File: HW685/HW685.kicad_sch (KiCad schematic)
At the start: 15 parts, among them J1 Screw_Terminal_01x03, J2 Screw_Terminal_01x02, U1 ICL7660, U2 LM358

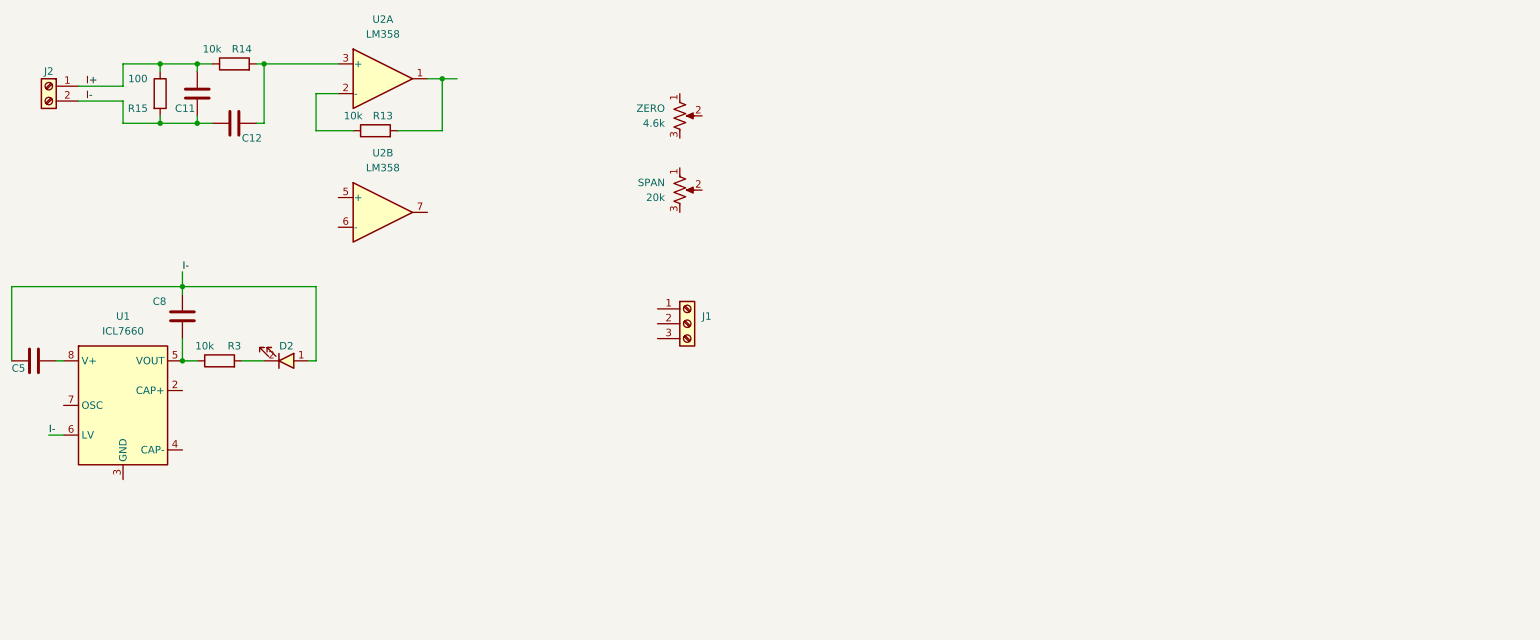
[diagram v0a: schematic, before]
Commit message: Complete HW685 Schematic
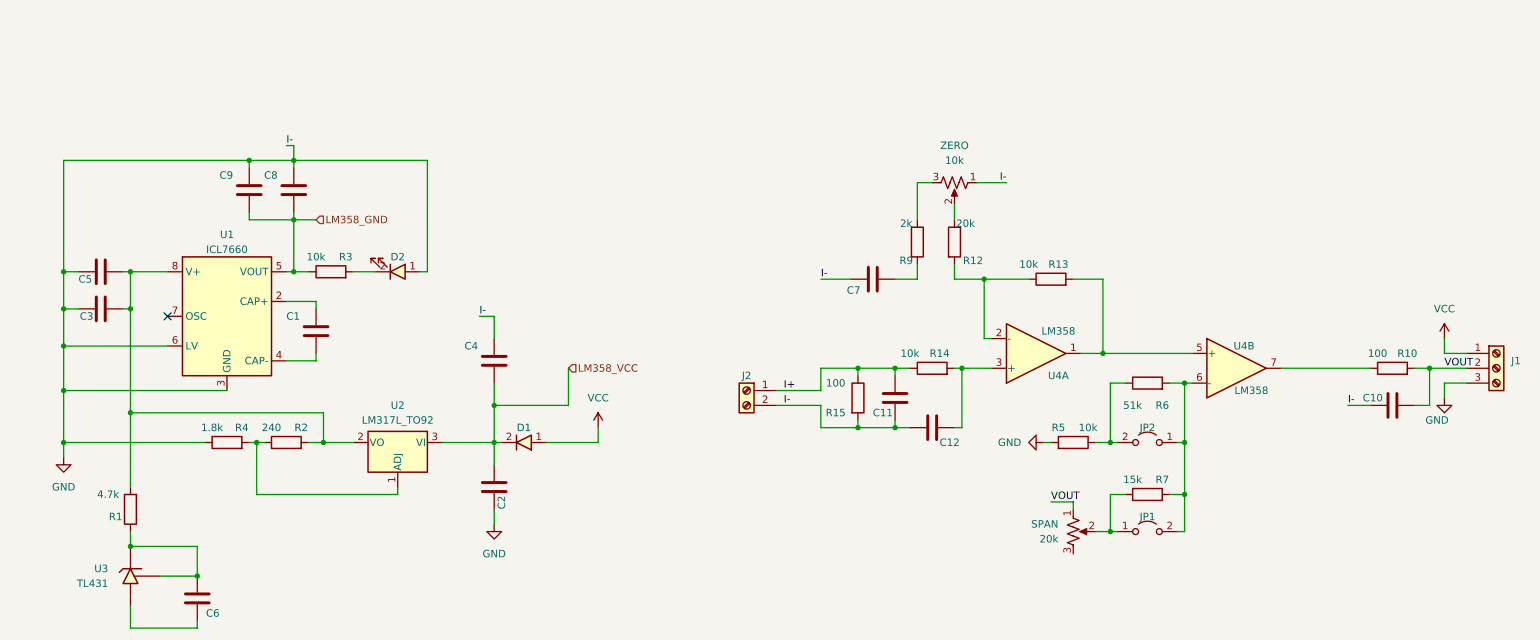
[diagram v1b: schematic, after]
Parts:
- added C1, C10, C2, C3, C4, C6, C7, C9: 10uF, symbol Device:C
- added D1: D_Diode, IVS_FOOTPRINTS:D_SMA, symbol IVS_SYMBOLS:D_Diode
- added JP1, JP2: Jumper_2_Open, symbol Jumper:Jumper_2_Open
- added R1: 4.7k, symbol Device:R
- added R10: 100, symbol Device:R
- added R12: 20k, symbol Device:R
- added R2: 240, symbol Device:R
- added R4: 1.8k, symbol Device:R
- added R5: 10k, symbol Device:R
- added R6: 51k, symbol Device:R
- added R7: 15k, symbol Device:R
- added R9: 2k, symbol Device:R
- added U2: LM317L_TO92, Package_TO_SOT_THT:TO-92_Inline, symbol Regulator_Linear:LM317L_TO92
- added U3: TL431, IVS_FOOTPRINTS:SOT23-3, symbol IVS_SYMBOLS:TL431
- ZERO: value 4.6k -> 10k
- renumbered U2 to U4
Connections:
- net I- is gone; now on net GND: C11.2, C12.2, C5.2, C8.1, D2.1, J2.2 (Pin_2), R15.2, U1.6 (LV)
- net at U1.2 (CAP+): now also C1.1
- net GND: now reaches U1.3 (GND)
- net GND: now also J1.3 (Pin_3), ZERO.1, C10.2, C2.2, C3.1, C4.1, C7.2, C9.1, R4.1, R5.2
- net at U1.4 (CAP-): now also C1.2
- net LM358_GND: now reaches C8.2, R3.1, U1.5 (VOUT)
- net LM358_GND: now also C9.2
- net at C5.1, U1.8 (V+): now also C3.2, R1.2, R2.2, U2.2 (VO)
- net VCC: now reaches J1.1 (Pin_1)
- net VCC: now also D1.1
- net VOUT: now reaches J1.2 (Pin_2)
- net VOUT: now also SPAN.1, C10.1, R10.2
- net at U4.5 (+): now also R13.2, U4.1
- net at U4.6 (-): now also JP1.2 (B), JP2.1 (A), R6.2, R7.2
- net at U4.7: now also R10.1
- net at R13.1, U4.2 (-): now also R12.2
- net at SPAN.2: now also JP1.1 (A), R7.1
- net at ZERO.2: now also R12.1
- net at ZERO.3: now also R9.1
- new net: JP2.2 (B), R5.1, R6.1
- new net: C6.1, R1.1, U3.1 (K), U3.2 (REF)
- new net: C6.2, U3.3 (A)
- new net: R2.1, R4.2, U2.1 (ADJ)
- new net: C7.1, R9.2
- new net LM358_VCC: C2.1, C4.2, D1.2, U2.3 (VI)
- no-connect marks 0 -> 1
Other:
- moved on the sheet: C11, C12, C5, C8, D2, J1, J2, R13, R14, R15, R3, SPAN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
